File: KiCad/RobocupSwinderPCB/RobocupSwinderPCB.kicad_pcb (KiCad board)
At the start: 2 copper layers, 92.4 x 57.4 mm, 30 parts, among them J1 Barrel_Jack, M1 Stepper_Motor_bipolar, M2 Stepper_Motor_bipolar, SW1 Limit_Switch, SW2 Limit_Switch, SW3 SW_SPST, U1 Teensy4.1, U3 LM7805_TO220

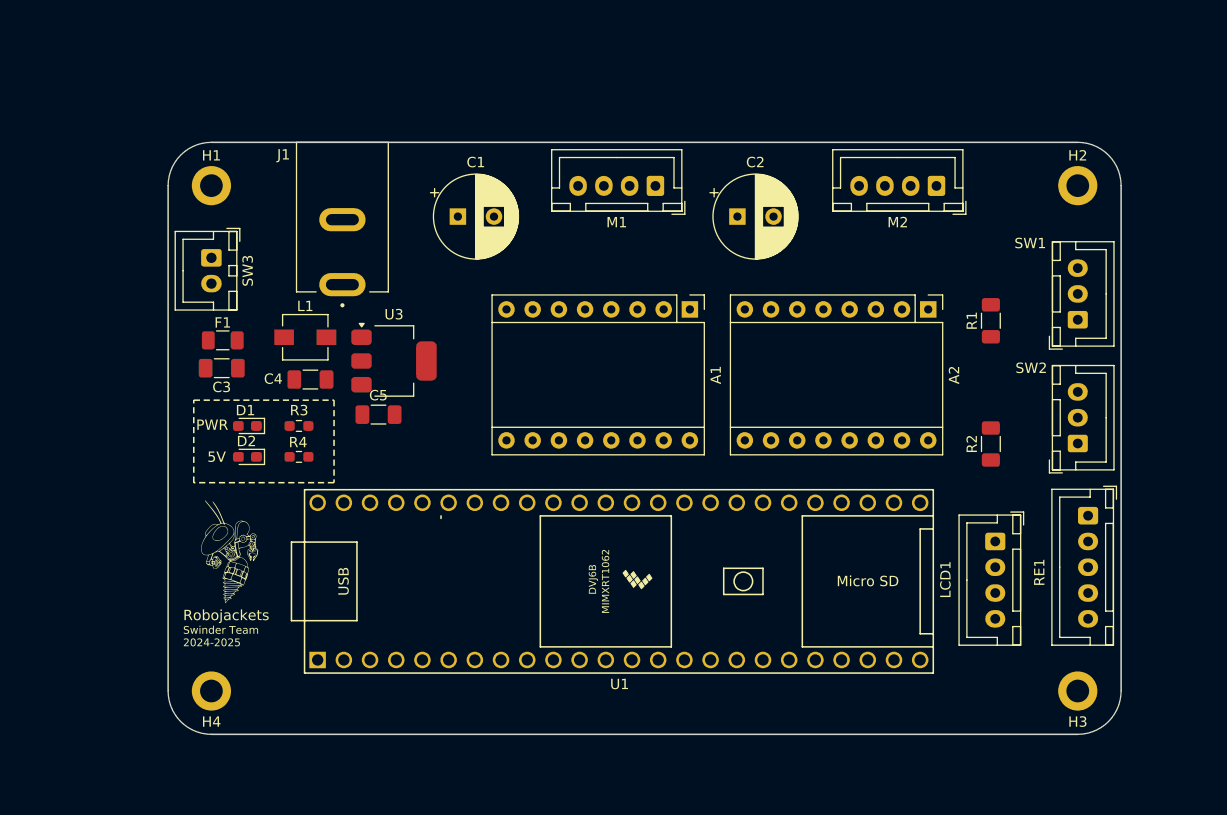
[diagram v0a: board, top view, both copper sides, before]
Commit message: Routing.
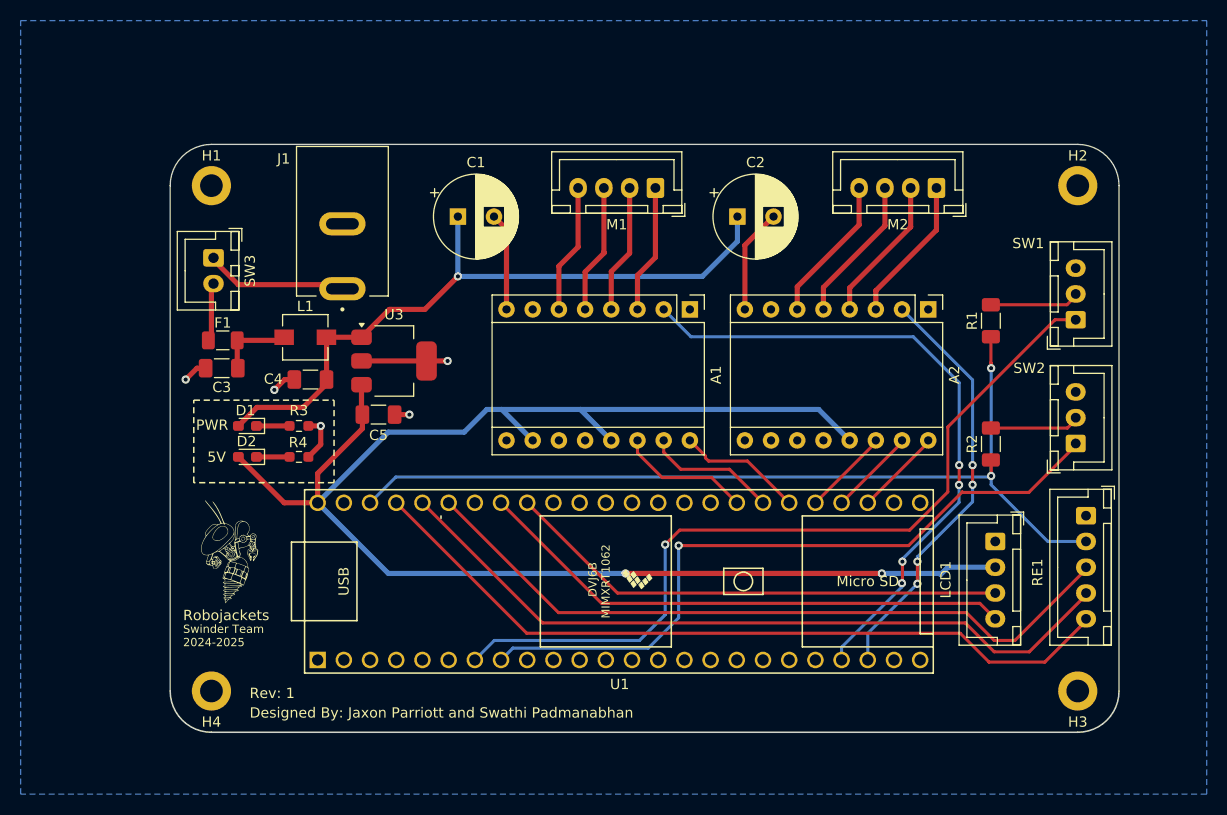
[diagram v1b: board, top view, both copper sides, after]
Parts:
- moved J1 0.40 mm to (106.2, 76.0)
- moved SW3 0.20 mm to (93.7, 73.0)
- moved M1 0.20 mm to (136.6, 66.2)
- moved M2 0.20 mm to (163.8, 66.2)
- moved RE1 0.20 mm to (178.3, 98.0)
- moved SW1 0.20 mm to (177.3, 79.0)
- moved SW2 0.20 mm to (177.3, 91.0)
- turned R3 to 0 degrees
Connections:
- A1 pad 2: /Feed_FLT_Pin_22 -> /Feed_FLT_Pin_21
- A2 pad 2: /Coil_FLT_Pin_21 -> /Coil_FLT_Pin_22
- U1 pad 21: /Coil_FLT_Pin_21 -> /Feed_FLT_Pin_21
- U1 pad 22: /Feed_FLT_Pin_22 -> /Coil_FLT_Pin_22
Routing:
- net +5V: track 0.00 -> 156.7 mm, vias 0 -> 2
- net +3.3V: track 0.00 -> 88.9 mm, vias 0 -> 2
- net /LSStart_Pin_7: track 0.00 -> 79.8 mm, vias 0 -> 1
- net /RE_CLK_Pin_23: track 0.00 -> 75.2 mm
- net /RE_DT_Pin_22: track 0.00 -> 72.9 mm
- net /RE_SW_Pin_21: track 0.00 -> 70.5 mm
- net /LSEnd_Pin_8: track 0.00 -> 68.8 mm, vias 0 -> 1
- net VCC: track 0.00 -> 67.2 mm, vias 0 -> 1
- net /Feed_FLT_Pin_21: track 0.00 -> 63.2 mm, vias 0 -> 4
- net /LCD_SCL_Pin_19: track 0.00 -> 52.6 mm
- net /LCD_SDA_Pin_18: track 0.00 -> 49.0 mm
- net /Coil_FLT_Pin_22: track 0.00 -> 41.1 mm, vias 0 -> 4
- net GND: track 0.00 -> 19.2 mm, vias 0 -> 5
- net Net-(A2-A2): track 0.00 -> 15.1 mm
- net Net-(A2-B2): track 0.00 -> 14.5 mm
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- added copper zone on B.Cu, net GND
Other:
- board size 92.4 x 57.4 mm -> 92 x 57 mm
- board text added: "49mm"
- board text added: "57mm"
- board text added: "84mm"
- board text added: "92mm"
- board text added: "Designed By: Jaxon Parriott and Swathi Padmanabhan"
- board text added: "Rev: 1"
